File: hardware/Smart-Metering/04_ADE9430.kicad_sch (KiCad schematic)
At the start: 14 parts, among them U1 ADE9430ACPZ, Y1 24.576MHz

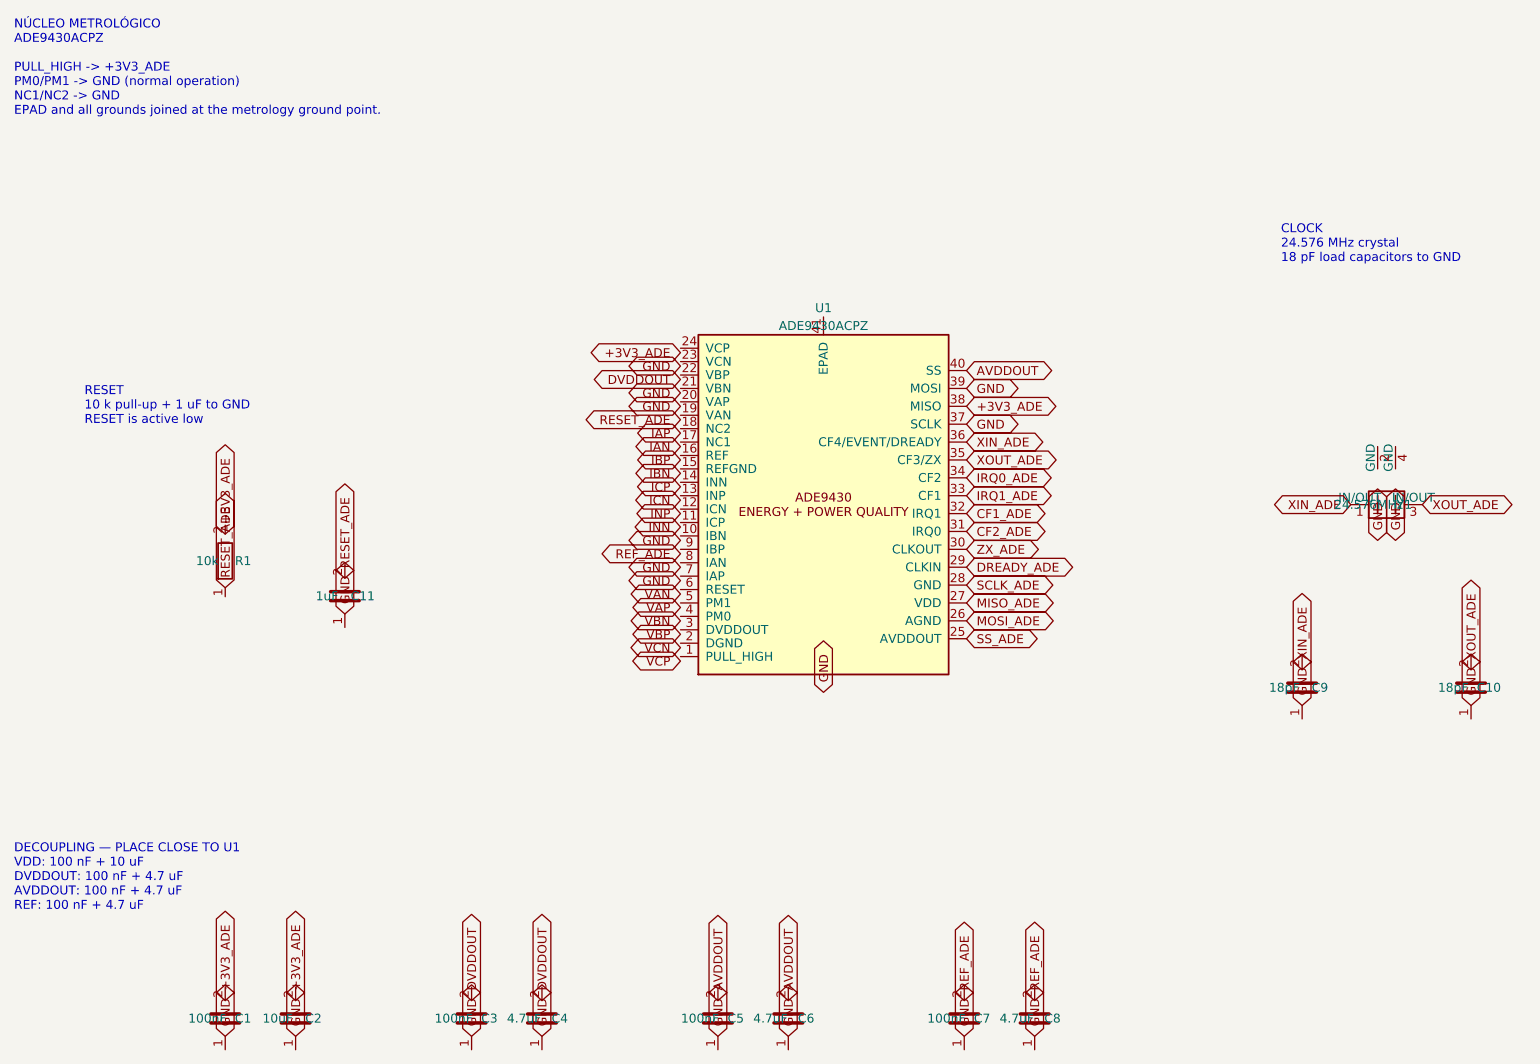
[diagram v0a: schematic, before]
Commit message: Alterações locais: folha 10 e ajustes nas folhas
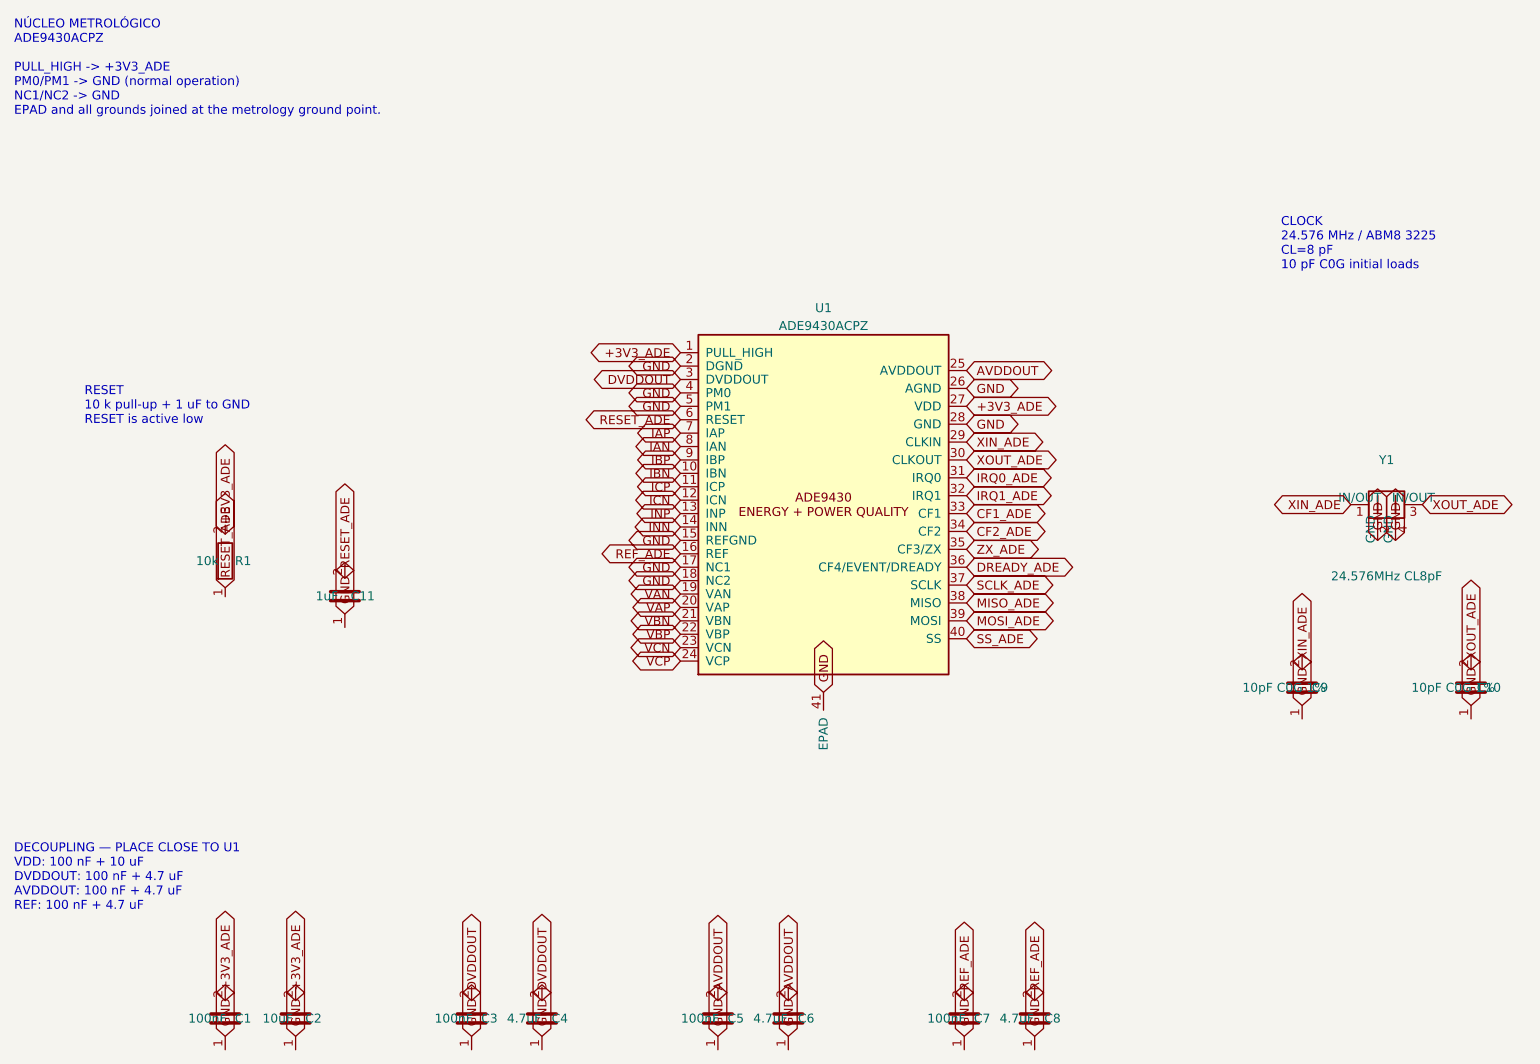
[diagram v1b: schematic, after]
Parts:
- C10, C9: value 18pF -> 10pF C0G 1%
- Y1: value 24.576MHz -> 24.576MHz CL8pF; MPN (none) -> ABM8-24.576MHZ-8-D1X-T
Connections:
- net +3V3_ADE: now also U1.1 (PULL_HIGH), U1.27 (VDD); no longer U1.38 (MISO)
- net AVDDOUT: now also U1.25 (AVDDOUT); no longer U1.40 (SS)
- net CF1_ADE: now also U1.33 (CF1); no longer U1.32 (IRQ1)
- net CF2_ADE: now also U1.34 (CF2); no longer U1.31 (IRQ0)
- net DREADY_ADE: now also U1.36 (CF4/EVENT/DREADY); no longer U1.29 (CLKIN)
- net DVDDOUT: now also U1.3 (DVDDOUT)
- net GND: now also U1.15 (REFGND), U1.17 (NC1), U1.18 (NC2), U1.2 (DGND), U1.26 (AGND), U1.28 (GND), U1.4 (PM0), U1.41 (EPAD), U1.5 (PM1), Y1.2 (GND), Y1.4 (GND); no longer U1.37 (SCLK), U1.39 (MOSI)
- net IAN: now also U1.8 (IAN)
- net IAP: now also U1.7 (IAP)
- net IBN: now also U1.10 (IBN)
- net IBP: now also U1.9 (IBP)
- net ICN: now also U1.12 (ICN)
- net ICP: now also U1.11 (ICP)
- net INN: now also U1.14 (INN)
- net INP: now also U1.13 (INP)
- net IRQ0_ADE: now also U1.31 (IRQ0); no longer U1.34 (CF2)
- net IRQ1_ADE: now also U1.32 (IRQ1); no longer U1.33 (CF1)
- net MISO_ADE: now also U1.38 (MISO); no longer U1.27 (VDD)
- net MOSI_ADE: now also U1.39 (MOSI); no longer U1.26 (AGND)
- net REF_ADE: now also U1.16 (REF)
- net RESET_ADE: now also U1.6 (RESET)
- net SCLK_ADE: now also U1.37 (SCLK); no longer U1.28 (GND)
- net SS_ADE: now also U1.40 (SS); no longer U1.25 (AVDDOUT)
- net VAN: now also U1.19 (VAN)
- net VAP: now also U1.20 (VAP)
- net VBN: now also U1.21 (VBN)
- net VBP: now also U1.22 (VBP)
- net VCN: now also U1.23 (VCN)
- net VCP: now also U1.24 (VCP)
- net XIN_ADE: now also U1.29 (CLKIN); no longer U1.36 (CF4/EVENT/DREADY)
- net XOUT_ADE: now also U1.30 (CLKOUT); no longer U1.35 (CF3/ZX)
- net ZX_ADE: now also U1.35 (CF3/ZX); no longer U1.30 (CLKOUT)
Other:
- note added: "CLOCK 24.576 MHz / ABM8 3225 CL=8 pF 10 pF C0G initial loads"
- note removed: "CLOCK 24.576 MHz crystal 18 pF load capacitors to GND"
- moved on the sheet: U1, Y1
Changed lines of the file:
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@@
 		(effects (font (size 1.27 1.27)) (justify left))
 	)
-	(text "CLOCK\n24.576 MHz crystal\n18 pF load capacitors to GND"
+	(text "CLOCK\n24.576 MHz / ABM8 3225\nCL=8 pF\n10 pF C0G initial loads"
 		(exclude_from_sim no)(at 205 55 0)
 		(effects (font (size 1.27 1.27)) (justify left))
@@
 		(unit 1)(body_style 1)
 		(exclude_from_sim no)(in_bom yes)(on_board yes)(in_pos_files yes)(dnp no)
-		(property "Reference" "Y1" (at 222.54 92 0) (effects (font (size 1.27 1.27))))
-		(property "Value" "24.576MHz" (at 217.46 92 0) (effects (font (size 1.27 1.27))))
+		(property "Reference" "Y1" (at 220 85.65 0) (effects (font (size 1.27 1.27))))
+		(property "Value" "24.576MHz CL8pF" (at 220 102.16 0) (effects (font (size 1.27 1.27))))
 		(property "Footprint" "Crystal:Crystal_SMD_3225-4Pin_3.2x2.5mm" (at 220 92 0) (effects (font (size 1.27 1.27)) (hide yes)))
-		(property "Datasheet" "" (at 220 92 0) (effects (font (size 1.27 1.27)) (hide yes)))
-		(property "Description" "ADE9430 master crystal, 24.576 MHz" (at 220 92 0) (effects (font (size 1.27 1.27)) (hide yes)))
+		(property "Datasheet" "https://abracon.com/Resonators/abm8.pdf" (at 220 92 0) (effects (font (size 1.27 1.27)) (hide yes)))
+		(property "MPN" "ABM8-24.576MHZ-8-D1X-T" (at 220 92 0) (effects (font (size 1.27 1.27)) (hide yes)))
+		(property "Description" "ABM8-24.576MHZ-8-D1X-T candidate; confirm orderability; ESR<=50ohm, C0<=3pF" (at 220 92 0) (effects (font (size 1.27 1.27)) (hide yes)))
 		(pin "1")
 		(pin "2")
@@
 		(exclude_from_sim no)(in_bom yes)(on_board yes)(in_pos_files yes)(dnp no)
 		(property "Reference" "C9" (at 210.54 118 0) (effects (font (size 1.27 1.27))))
-		(property "Value" "18pF" (at 205.46 118 0) (effects (font (size 1.27 1.27))))
+		(property "Value" "10pF C0G 1%" (at 205.46 118 0) (effects (font (size 1.27 1.27))))
 		(property "Footprint" "Capacitor_SMD:C_0603_1608Metric" (at 208 118 0) (effects (font (size 1.27 1.27)) (hide yes)))
 		(property "Datasheet" "" (at 208 118 0) (effects (font (size 1.27 1.27)) (hide yes)))
-		(property "Description" "Crystal load capacitor" (at 208 118 0) (effects (font (size 1.27 1.27)) (hide yes)))
+		(property "Description" "Initial load: CL8pF, Cin4pF and estimated Cp2pF per pin; verify PCB" (at 208 118 0) (effects (font (size 1.27 1.27)) (hide yes)))
 		(pin "1")
 		(pin "2")
@@
 		(exclude_from_sim no)(in_bom yes)(on_board yes)(in_pos_files yes)(dnp no)
 		(property "Reference" "C10" (at 234.54 118 0) (effects (font (size 1.27 1.27))))
-		(property "Value" "18pF" (at 229.46 118 0) (effects (font (size 1.27 1.27))))
+		(property "Value" "10pF C0G 1%" (at 229.46 118 0) (effects (font (size 1.27 1.27))))
 		(property "Footprint" "Capacitor_SMD:C_0603_1608Metric" (at 232 118 0) (effects (font (size 1.27 1.27)) (hide yes)))
 		(property "Datasheet" "" (at 232 118 0) (effects (font (size 1.27 1.27)) (hide yes)))
-		(property "Description" "Crystal load capacitor" (at 232 118 0) (effects (font (size 1.27 1.27)) (hide yes)))
-		(pin "1")
-		(pin "2")
+		(property "Description" "Initial load: CL8pF, Cin4pF and estimated Cp2pF per pin; verify PCB" (at 232 118 0) (effects (font (size 1.27 1.27)) (hide yes)))
+		(pin "1")
+		(pin "2")
